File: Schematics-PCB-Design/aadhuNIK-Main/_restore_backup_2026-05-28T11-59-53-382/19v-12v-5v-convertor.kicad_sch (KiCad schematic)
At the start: 19 parts, among them J6 Barrel_Jack, J7 Conn_01x01_Pin, J8 Conn_01x01_Pin, U13 LM2596S-5, U14 LM2596S-ADJ

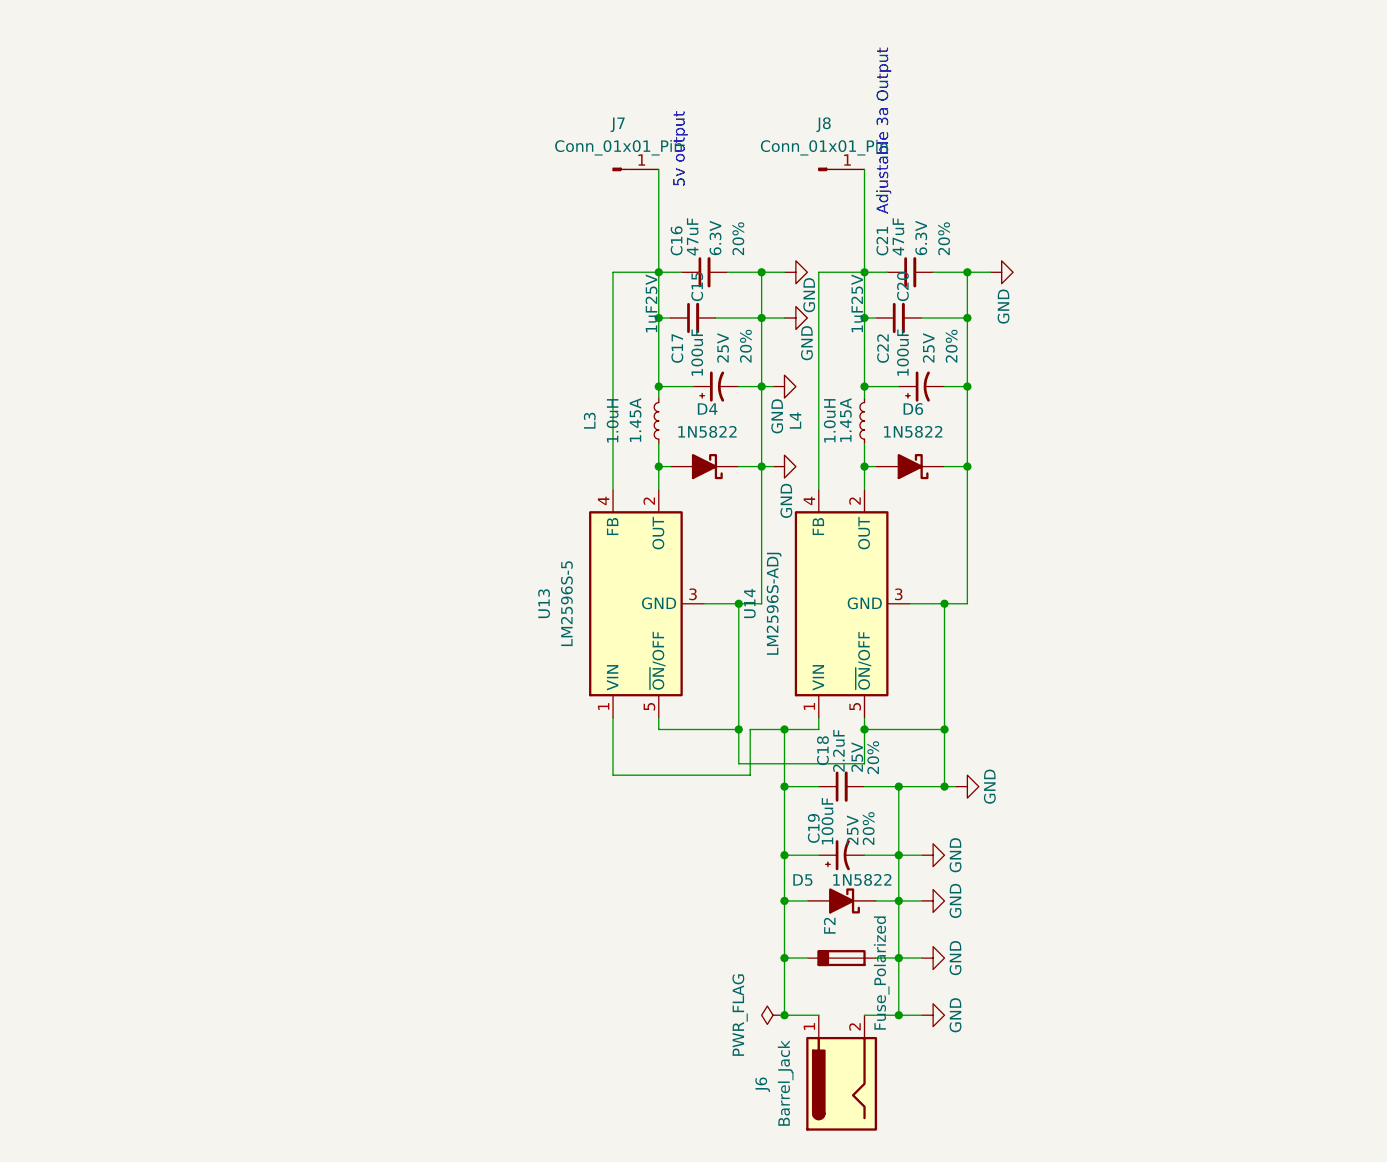
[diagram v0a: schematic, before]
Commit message: Update KiCad schematic and PCB
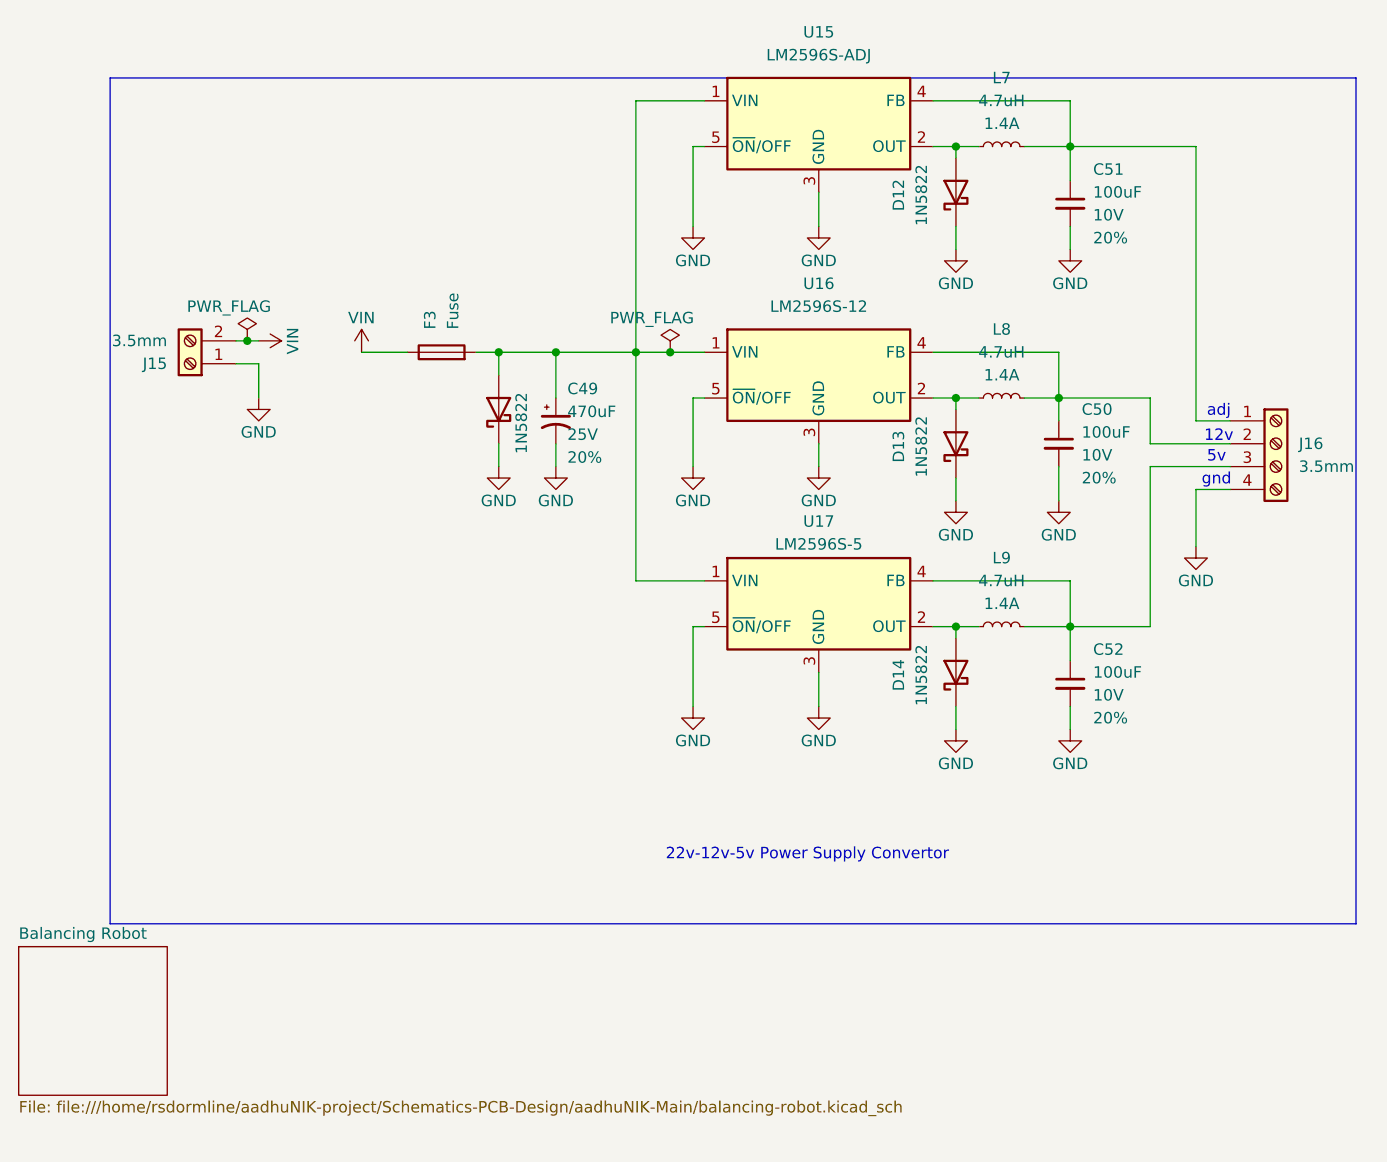
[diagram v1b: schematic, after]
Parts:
- removed C15, C20: 1uF_0603_25V, PCM_4ms_Capacitor:C_0603, symbol PCM_4ms_Capacitor:1uF_0603_25V
- removed C16, C21: 47uF, PCM_SparkFun-Capacitor:C_0805_2012Metric, symbol PCM_SparkFun-Capacitor:47uF_0805_6.3V_20%
- removed C17, C19, C22: 100uF, PCM_SparkFun-Capacitor:Panasonic_D, symbol PCM_SparkFun-Capacitor:100uF_6.6x6.6_25V_20%
- removed C18: 2.2uF, PCM_SparkFun-Capacitor:C_0805_2012Metric, symbol PCM_SparkFun-Capacitor:2.2uF_0805_25V_20%
- removed D4, D5, D6: 1N5822, PCM_Diode_THT_AKL:D_DO-201AD_P12.70mm_Horizontal, symbol PCM_Diode_Schottky_AKL:1N5822
- removed F2: Fuse_Polarized, Fuse:Fuse_0402_1005Metric, symbol Device:Fuse_Polarized
- removed J6: Barrel_Jack, Connector_BarrelJack:BarrelJack_SwitchcraftConxall_RAPC10U_Horizontal, symbol Connector:Barrel_Jack
- removed J7, J8: Conn_01x01_Pin, Connector_PinHeader_1.00mm:PinHeader_1x01_P1.00mm_Vertical, symbol Connector:Conn_01x01_Pin
- removed L3, L4: 1.0uH, PCM_SparkFun-Coil:0805, symbol PCM_SparkFun-Coil:1.0uH_0805_1.45A
- removed U13: LM2596S-5, PCM_Package_TO_SOT_SMD_AKL:TO-263-4_ThermalVias, symbol Regulator_Switching:LM2596S-5
- removed U14: LM2596S-ADJ, Package_TO_SOT_SMD:TO-263-5_TabPin3, symbol Regulator_Switching:LM2596S-ADJ
- added C49: 470uF, PCM_SparkFun-Capacitor:Electrolytic_10.3x10.3mm, symbol PCM_SparkFun-Capacitor:470uF_10x10_25V_20%
- added C50, C51, C52: 100uF, PCM_SparkFun-Capacitor:C_1206_3216Metric, symbol PCM_SparkFun-Capacitor:100uF_1206_50V_10%
- added D11, D12, D13, D14: 1N5822, Diode_THT:D_DO-201AD_P15.24mm_Horizontal, symbol Diode:1N5822
- added F3: Fuse, Fuse:Fuse_0603_1608Metric, symbol Device:Fuse
- added J15: 3.5mm, PCM_SparkFun-Connector:ScrewTerminal_1x02_P3.5mm_Horizontal_Black, symbol PCM_SparkFun-Connector:ScrewTerminal_1x02_P3.5mm_Horizontal_Black
- added J16: 3.5mm, PCM_SparkFun-Connector:ScrewTerminal_1x04_P3.5mm_Horizontal, symbol PCM_SparkFun-Connector:ScrewTerminal_1x04_P3.5mm_Horizontal
- added L7, L8, L9: 4.7uH, PCM_SparkFun-Coil:1008_2520Metric, symbol PCM_SparkFun-Coil:4.7uH_1008_1.4A
- added U15: LM2596S-ADJ, Package_TO_SOT_SMD:TO-263-5_TabPin3, symbol Regulator_Switching:LM2596S-ADJ
- added U16: LM2596S-12, Package_TO_SOT_SMD:TO-263-5_TabPin3, symbol Regulator_Switching:LM2596S-12
- added U17: LM2596S-5, Package_TO_SOT_SMD:TO-263-5_TabPin3, symbol Regulator_Switching:LM2596S-5
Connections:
- net GND: now also C49.2, C50.2, C51.2, C52.2, D11.1 (K), D12.1 (K), D13.1 (K), D14.1 (K), J15.1 (Pin_1), J16.4 (Pin_4), U15.3 (GND), U15.5 (~{ON}/OFF), U16.3 (GND), U16.5 (~{ON}/OFF), U17.3 (GND), U17.5 (~{ON}/OFF)
- new net: C49.1, D11.2 (A), F3.2, U15.1 (VIN), U16.1 (VIN), U17.1 (VIN)
- new net: D13.2 (A), L8.1, U16.2 (OUT)
- new net: D14.2 (A), L9.1, U17.2 (OUT)
- new net: C52.1, J16.3 (Pin_3), L9.2, U17.4 (FB)
- new net: D12.2 (A), L7.1, U15.2 (OUT)
- new net: C51.1, J16.1 (Pin_1), L7.2, U15.4 (FB)
- new net: C50.1, J16.2 (Pin_2), L8.2, U16.4 (FB)
- new net VIN: F3.1, J15.2 (Pin_2)
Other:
- added sheet Balancing Robot (file:///home/rsdormline/aadhuNIK-project/Schematics-PCB-Design/aadhuNIK-Main/balancing-robot.kicad_sch)
- note added: "12v"
- note added: "22v-12v-5v Power Supply Convertor"
- note added: "5v"
- note added: "adj"
- note added: "gnd"
- note removed: "5v output"
- note removed: "Adjustable 3a Output"
